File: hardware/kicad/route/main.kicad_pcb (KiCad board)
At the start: 2 copper layers, 150 x 100 mm, 43 parts, among them P1 CONN_02X20, U1 74LS245, U2 74LS245

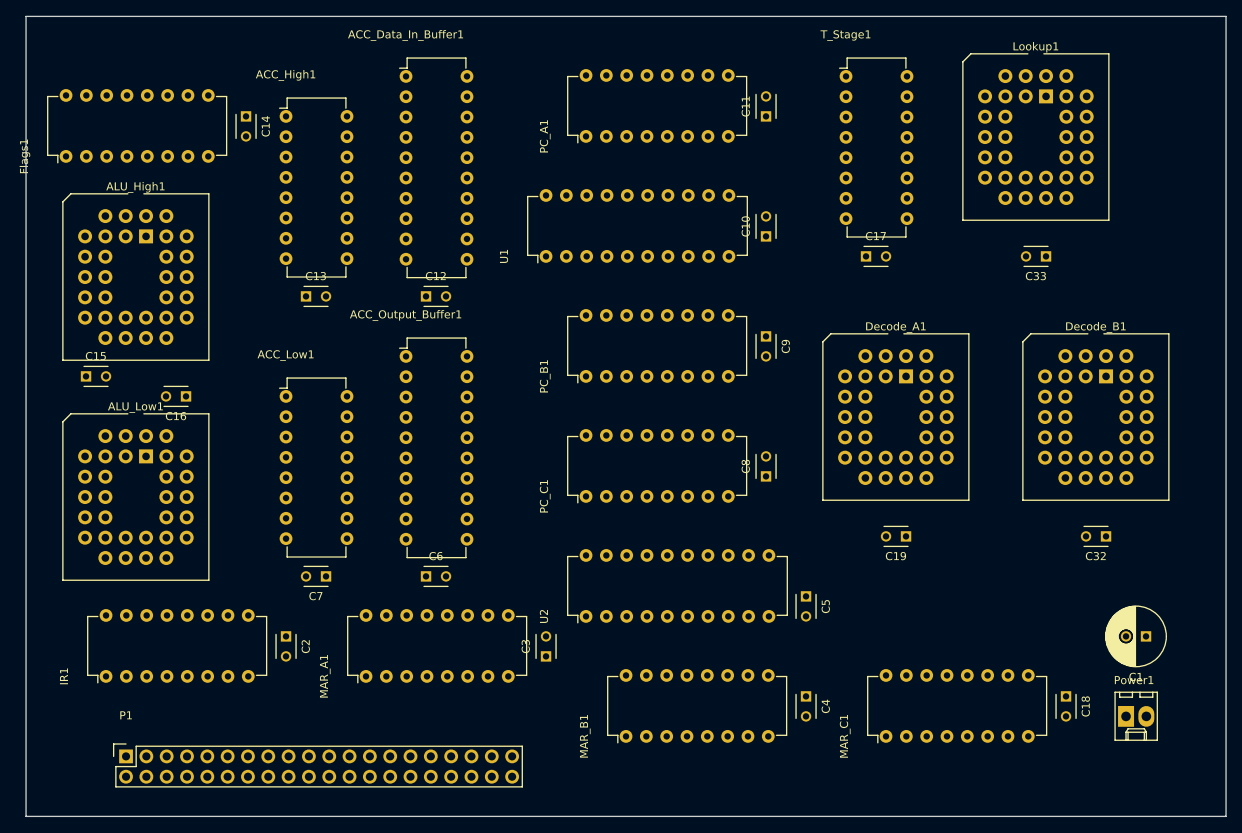
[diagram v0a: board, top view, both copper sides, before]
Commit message: Just a backup.
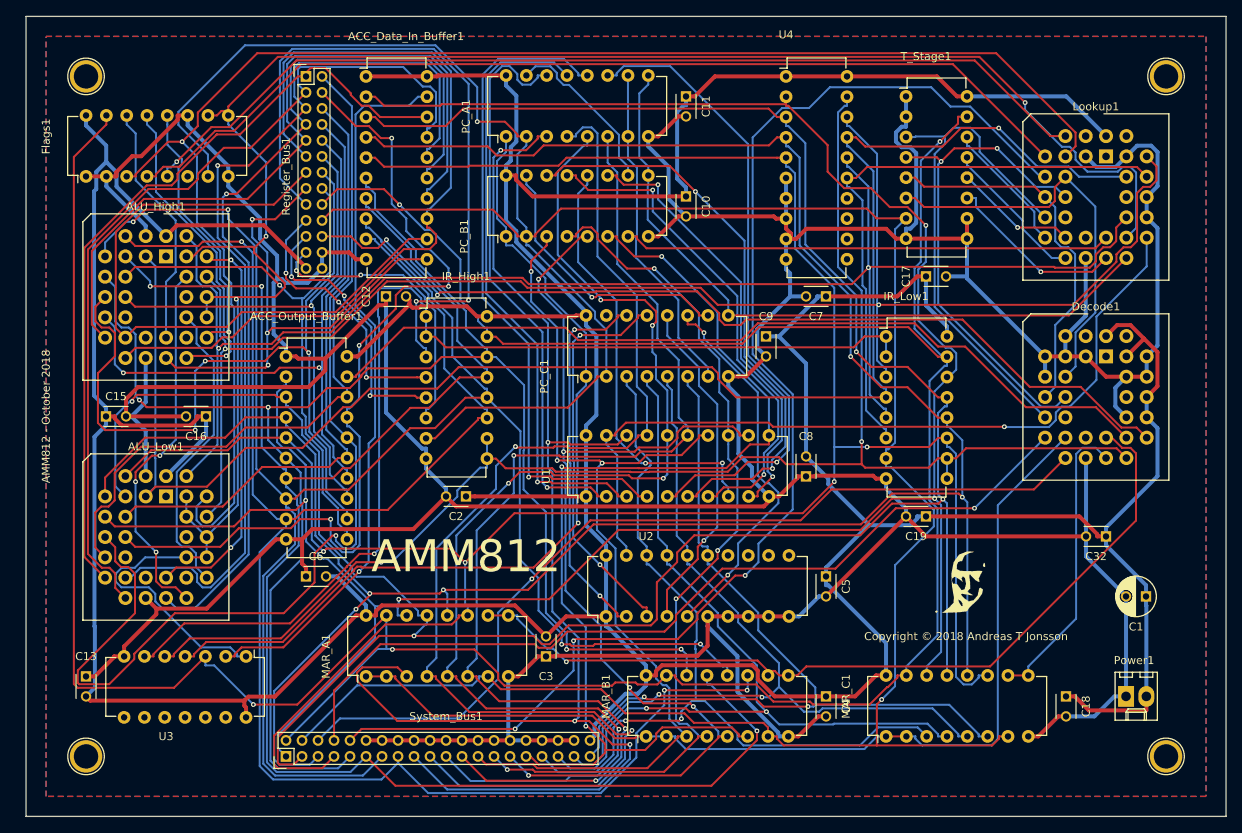
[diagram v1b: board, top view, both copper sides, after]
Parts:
- removed ACC_High1, ACC_Low1, IR1: 74LS173, Housings_DIP:DIP-16_W7.62mm
- removed C14, C33: 100nF, Capacitors_ThroughHole:C_Disc_D3_P2.5
- removed Decode_A1, Decode_B1: AT28HC64BF, PLCC32_bugfix:PLCC-32_THT-Socket_bugfix
- removed P1: CONN_02X20, Socket_Strips:Socket_Strip_Straight_2x20
- added Decode1: AT28HC64BF, PLCC32_bugfix:PLCC-32_THT-Socket_bugfix, F.Cu at (195.0, 102.5)
- added G***: LOGO, Logo:logo, F.Cu at (177.5, 130.0)
- added IR_High1: 74LS173, Housings_DIP:DIP-16_W7.62mm, F.Cu at (110.0, 97.5)
- added IR_Low1: 74LS173, Housings_DIP:DIP-16_W7.62mm, F.Cu at (167.5, 100.0)
- added REF1: 1pin, Connect:1pin, F.Cu at (67.5, 67.5)
- added REF2: 1pin, Connect:1pin, F.Cu at (202.5, 67.5)
- added REF3: 1pin, Connect:1pin, F.Cu at (202.5, 152.5)
- added REF4: 1pin, Connect:1pin, F.Cu at (67.5, 152.5)
- added Register_Bus1: CONN_02X13, Pin_Headers:Pin_Header_Straight_2x13_Pitch2.00mm, F.Cu at (95.0, 67.5)
- added System_Bus1: CONN_02X20, Pin_Headers:Pin_Header_Straight_2x20_Pitch2.00mm, F.Cu at (92.5, 152.5)
- added U3: 74LS04, Housings_DIP:DIP-14_W7.62mm, F.Cu at (87.5, 140.0)
- added U4: 74LS245, Housings_DIP:DIP-20_W7.62mm, F.Cu at (155.0, 67.5)
- C1: footprint Capacitors_ThroughHole:C_Radial_D7.5_L11.2_P2.5 -> Capacitors_ThroughHole:C_Radial_D5_L11_P2.5
- moved C7 71.6 mm to (160.0, 95.0)
- moved C13 54.9 mm to (67.5, 142.5), turned to 270 degrees
- moved U1 30.4 mm to (130.0, 120.0)
- moved C2 28.5 mm to (115.0, 120.0), turned to 180 degrees
- moved PC_B1 20.2 mm to (120.0, 87.5)
- moved ACC_Output_Buffer1 15.0 mm to (92.5, 102.5)
- moved C6 15.0 mm to (95.0, 130.0)
- moved PC_C1 15.0 mm to (130.0, 105.0)
- moved C10 11.2 mm to (142.5, 82.5), turned to 270 degrees
- moved Lookup1 10.6 mm to (195.0, 77.5)
- moved C11 10.3 mm to (142.5, 70.0), turned to 270 degrees
- moved PC_A1 10.0 mm to (120.0, 75.0)
- moved C17 7.91 mm to (172.5, 92.5)
- moved T_Stage1 7.91 mm to (170.0, 70.0)
- moved ALU_Low1 5.59 mm to (77.5, 120.0)
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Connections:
- net Ctrl_MAR_Output renamed Ctrl_MAR_Output_I
- ACC_Data_In_Buffer1 pad 19: Ctrl_ACC_Source -> Net-(ACC_Data_In_Buffer1-Pad19)
- ACC_Output_Buffer1 pad 19: Ctrl_ACC_Output -> Ctrl_ACC_Output_I
- ALU_High1 pad 23: VCC -> Ctrl_ALU_Enable_I
- ALU_High1 pad 25: Ctrl_ALU_Enable -> Ctrl_ALU_Enable_I
- ALU_High1 pad 31: VCC -> Ctrl_ALU_Enable_I
- ALU_Low1 pad 23: VCC -> Ctrl_ALU_Enable_I
- ALU_Low1 pad 24: GND -> Ctrl_ALU_Enable_I
- ALU_Low1 pad 25: Ctrl_ALU_Enable -> Ctrl_ALU_Enable_I
- ALU_Low1 pad 28: GND -> Ctrl_ALU_Enable_I
- ALU_Low1 pad 31: VCC -> Ctrl_ALU_Enable_I
- C10 pad 1: GND -> VCC
- C10 pad 2: VCC -> GND
- C11 pad 1: GND -> VCC
- C11 pad 2: VCC -> GND
- Flags1 pad 10: Ctrl_ALU_Enable -> Ctrl_ALU_Enable_I
- Flags1 pad 9: Ctrl_ALU_Enable -> Ctrl_ALU_Enable_I
- Lookup1 pad 19: Net-(Decode_A1-Pad11) -> Ctrl_PC_Count
- Lookup1 pad 20: Net-(Decode_A1-Pad10) -> Ctrl_PC_Input_I
- Lookup1 pad 21: Net-(Decode_A1-Pad9) -> Ctrl_PC_Output_I
- Lookup1 pad 22: Net-(Decode_A1-Pad8) -> Ctrl_ALU_Enable_I
- Lookup1 pad 23: VCC -> GND
- Lookup1 pad 25: VCC -> GND
- Lookup1 pad 31: VCC -> GND
- MAR_A1 pad 10: Ctrl_MAR_Low_Input -> Ctrl_MAR_Low_Input_I
- MAR_A1 pad 11: Data7 -> Data3
- MAR_A1 pad 12: Data6 -> Data2
- MAR_A1 pad 13: Data5 -> Data1
- MAR_A1 pad 14: Data4 -> Data0
- MAR_A1 pad 9: Ctrl_MAR_Low_Input -> Ctrl_MAR_Low_Input_I
- MAR_B1 pad 10: Ctrl_MAR_High_Input -> Ctrl_MAR_Low_Input_I
- MAR_B1 pad 11: Data3 -> Data7
- MAR_B1 pad 12: Data2 -> Data6
- MAR_B1 pad 13: Data1 -> Data5
- MAR_B1 pad 14: Data0 -> Data4
- MAR_B1 pad 9: Ctrl_MAR_High_Input -> Ctrl_MAR_Low_Input_I
- MAR_C1 pad 10: Ctrl_MAR_High_Input -> Ctrl_MAR_High_Input_I
- MAR_C1 pad 11: Data7 -> Data3
- MAR_C1 pad 12: Data6 -> Data2
- MAR_C1 pad 13: Data5 -> Data1
- MAR_C1 pad 14: Data4 -> Data0
- MAR_C1 pad 9: Ctrl_MAR_High_Input -> Ctrl_MAR_High_Input_I
- PC_A1 pad 1: Reset -> Net-(PC_A1-Pad1)
- PC_A1 pad 9: Ctrl_PC_Input -> Ctrl_PC_Input_I
- PC_B1 pad 1: Reset -> Net-(PC_A1-Pad1)
- PC_B1 pad 9: Ctrl_PC_Input -> Ctrl_PC_Input_I
- PC_C1 pad 1: Reset -> Net-(PC_A1-Pad1)
- PC_C1 pad 9: Ctrl_PC_Input -> Ctrl_PC_Input_I
- U1 pad 19: Ctrl_PC_Output -> Ctrl_PC_Output_I
- U2 pad 19: Ctrl_PC_Output -> Ctrl_PC_Output_I
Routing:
- net GND: track 0.00 -> 722.2 mm
- net VCC: track 0.00 -> 695.6 mm
- net Reset: track 0.00 -> 386.0 mm, vias 0 -> 4
- net Clock: track 0.00 -> 371.9 mm, vias 0 -> 2
- net Data1: track 0.00 -> 317.5 mm, vias 0 -> 4
- net Data0: track 0.00 -> 305.7 mm, vias 0 -> 4
- net Data2: track 0.00 -> 303.3 mm, vias 0 -> 5
- net Data3: track 0.00 -> 303.0 mm, vias 0 -> 4
- net Ctrl_ALU_Enable_I: track 0.00 -> 258.0 mm, vias 0 -> 3
- net Data6: track 0.00 -> 227.1 mm, vias 0 -> 4
- net Data7: track 0.00 -> 220.2 mm, vias 0 -> 3
- net Data5: track 0.00 -> 219.0 mm, vias 0 -> 3
- net Data4: track 0.00 -> 211.1 mm, vias 0 -> 4
- net IR1: track 0.00 -> 206.0 mm, vias 0 -> 1
- net IR0: track 0.00 -> 202.1 mm, vias 0 -> 2
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- added copper zone on B.Cu, net GND
- added copper zone on F.Cu, net VCC
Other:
- net class GND added: clearance 0.2, trace_width 0.5, via_dia 1.2, via_drill 0.8
- net class VCC added: clearance 0.2, trace_width 0.5, via_dia 1.2, via_drill 0.8
- board text added: "AMM812"
- board text added: "AMM812 - October 2018"
- board text added: "Copyright © 2018 Andreas T Jonsson"
